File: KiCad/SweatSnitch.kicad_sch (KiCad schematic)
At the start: 5 parts, among them U1 HDC1080DMBR, U2 XIAO-RP2040-DIP

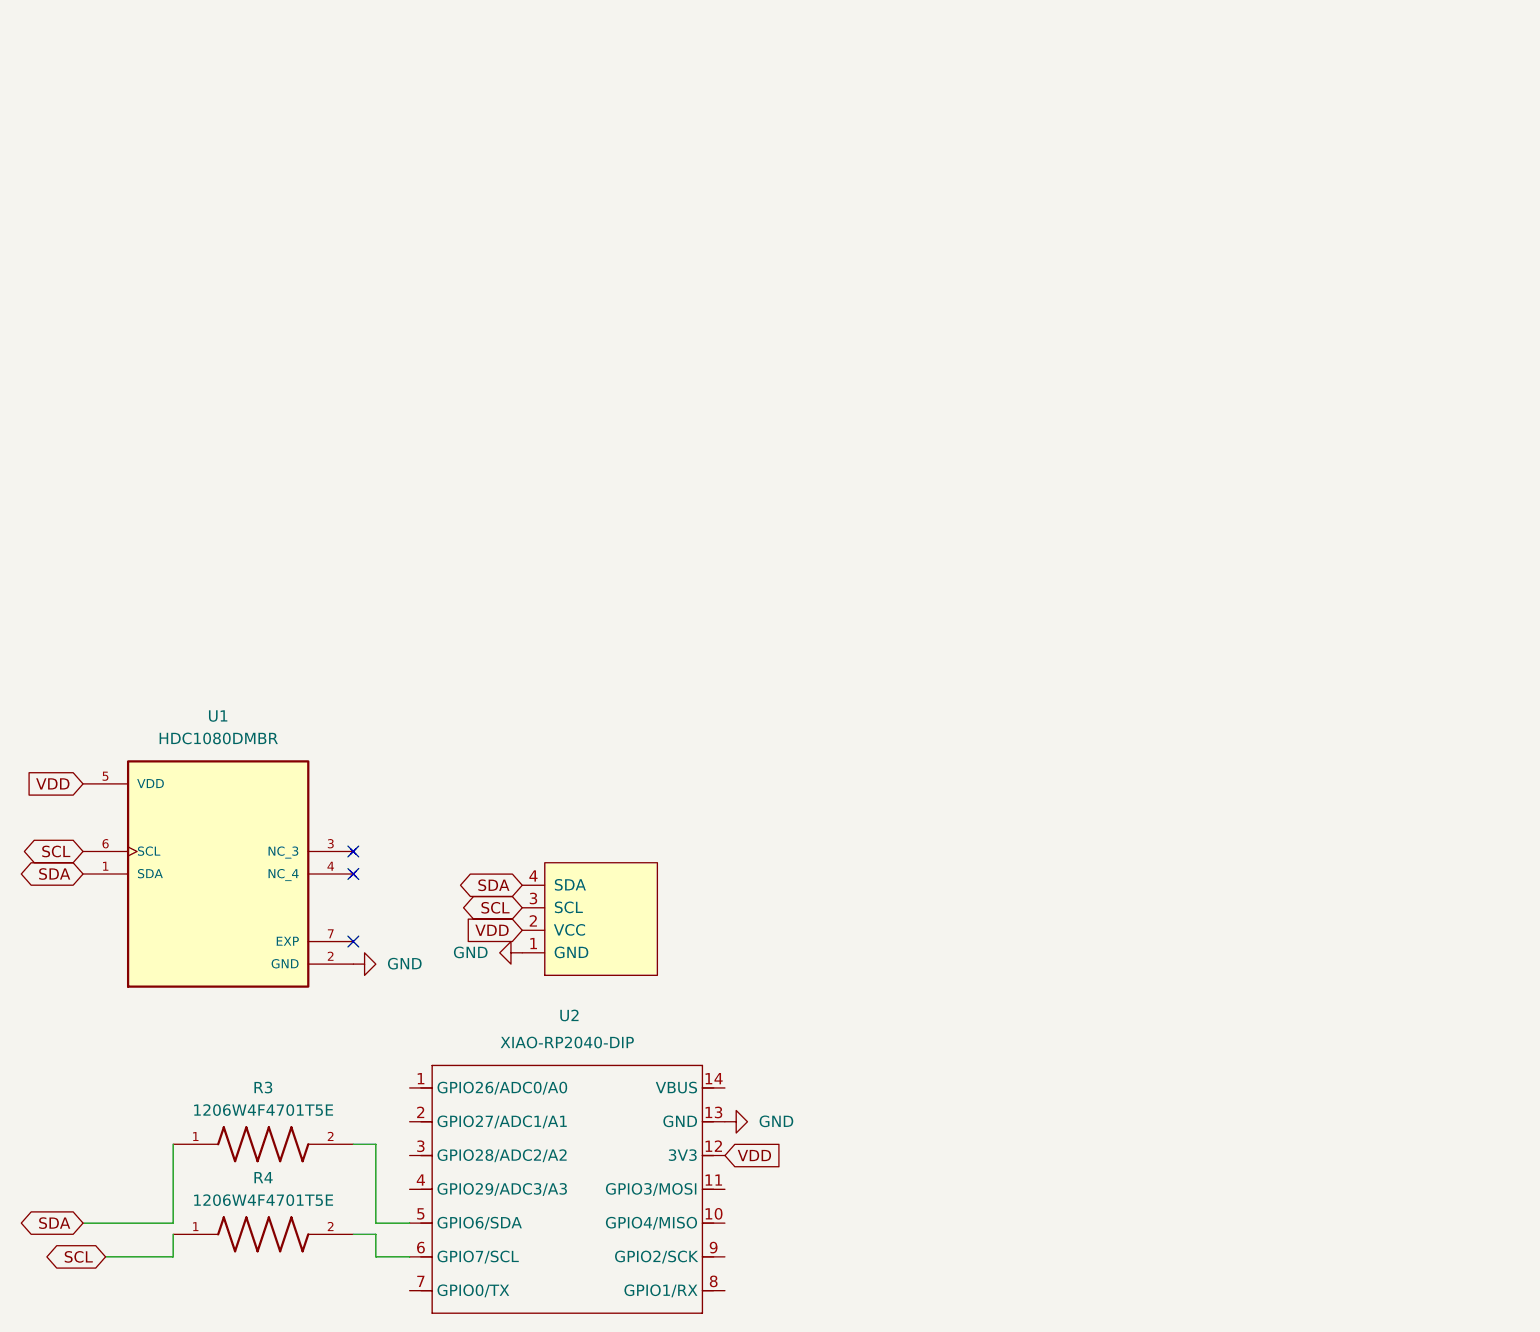
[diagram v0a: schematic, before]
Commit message: Add files via upload
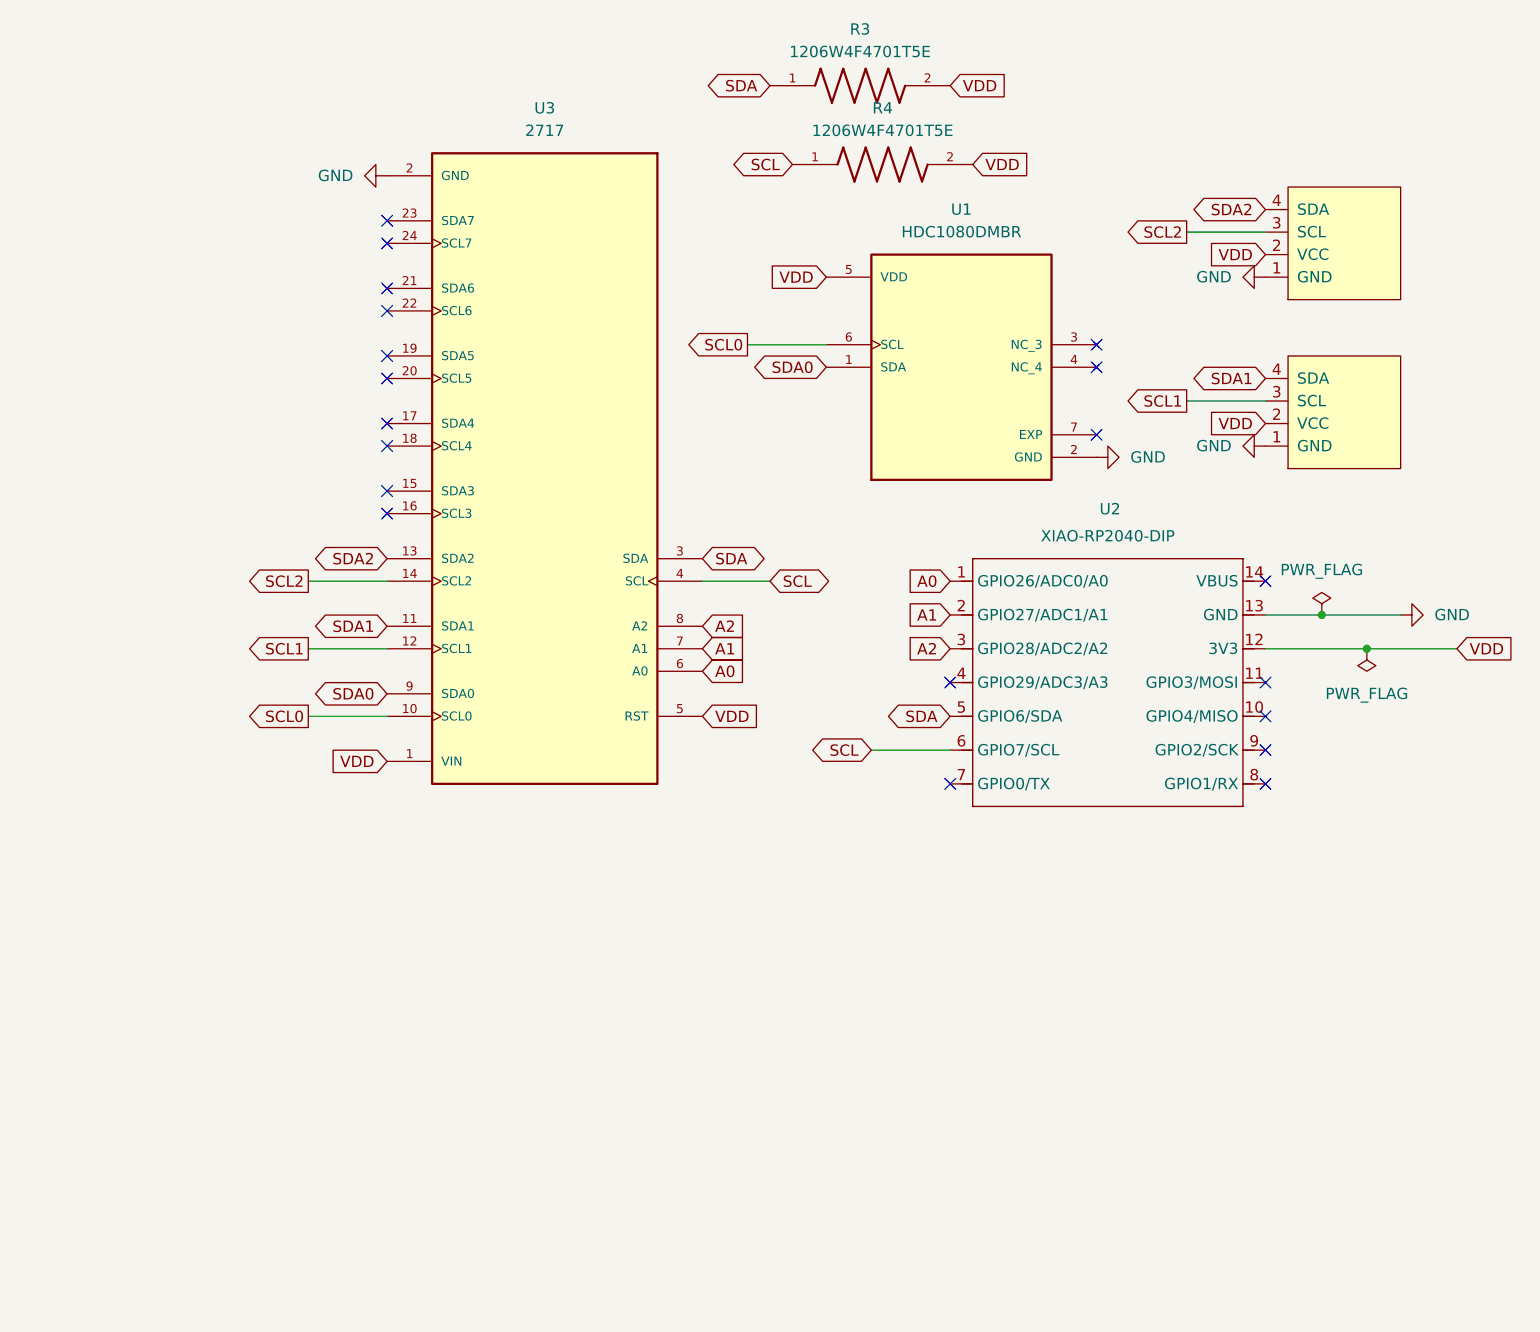
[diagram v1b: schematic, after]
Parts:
- added Brd2: SSD1306, oled:SSD1306-0.91-OLED-4pin-128x32, symbol SSD1306-128x64_OLED:SSD1306
- added U3: 2717, hii:MODULE_2717, symbol 2717:2717
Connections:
- net GND: now also Brd2.1 (GND), U3.2 (GND)
- net SCL: now also U2.6 (GPIO7/SCL), U3.4 (SCL); no longer Brd1.3 (SCL), U1.6 (SCL)
- net SDA: now also U2.5 (GPIO6/SDA), U3.3 (SDA); no longer Brd1.4 (SDA), U1.1 (SDA)
- net VDD: now also R3.2, R4.2, Brd2.2 (VCC), U3.1 (VIN), U3.5 (RST)
- net A0: now reaches U2.1 (GPIO26/ADC0/A0)
- net A0: now also U3.6 (A0)
- net A1: now reaches U2.2 (GPIO27/ADC1/A1)
- net A1: now also U3.7 (A1)
- net A2: now reaches U2.3 (GPIO28/ADC2/A2)
- net A2: now also U3.8 (A2)
- new net SCL0: U1.6 (SCL), U3.10 (SCL0)
- new net SCL1: Brd1.3 (SCL), U3.12 (SCL1)
- new net SCL2: Brd2.3 (SCL), U3.14 (SCL2)
- new net SDA0: U1.1 (SDA), U3.9 (SDA0)
- new net SDA1: Brd1.4 (SDA), U3.11 (SDA1)
- new net SDA2: Brd2.4 (SDA), U3.13 (SDA2)
- no-connect marks 3 -> 20
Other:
- moved on the sheet: R3, R4, U1, U2
